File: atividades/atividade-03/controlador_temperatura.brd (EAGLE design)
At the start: 68.6 x 53.3 mm, 34 parts, among them Q1 BC337, Q2 BC337, Q3 BC337

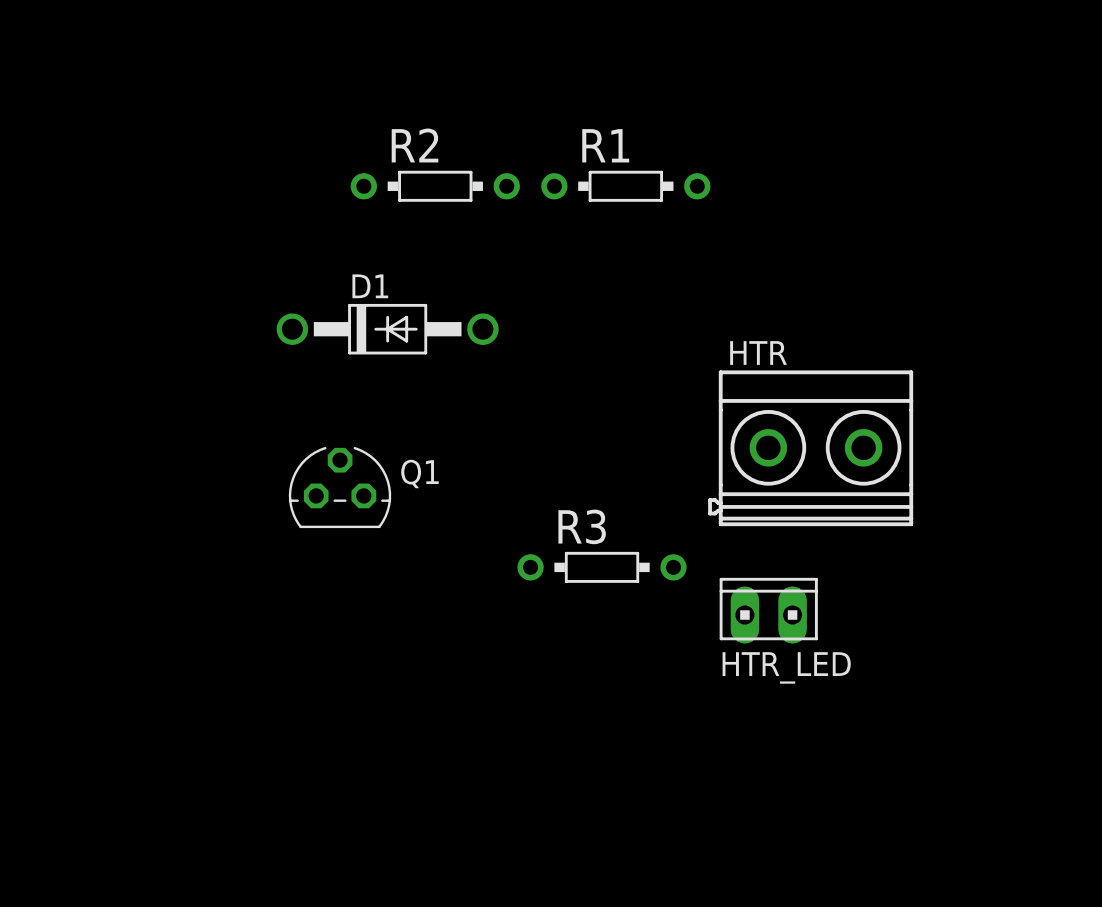
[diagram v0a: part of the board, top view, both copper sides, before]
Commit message: heater realinhado
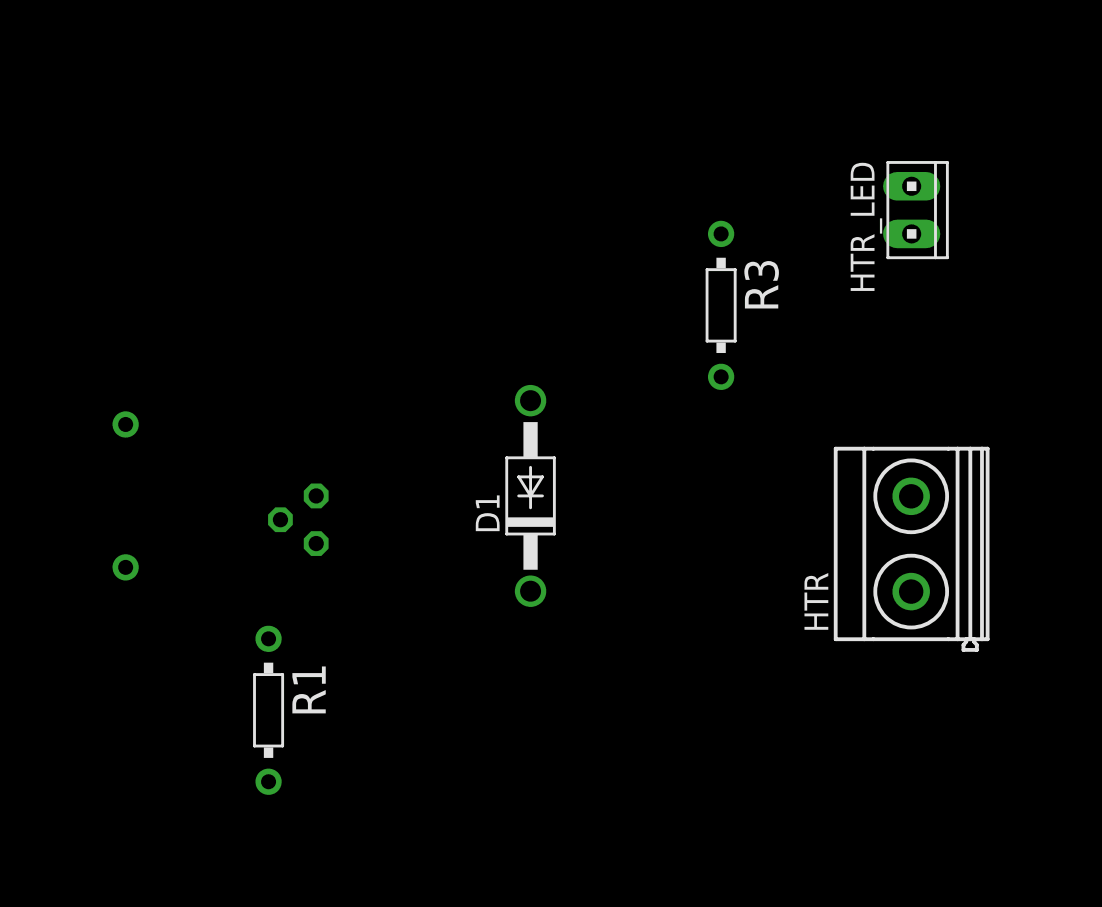
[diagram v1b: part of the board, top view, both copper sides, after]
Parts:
- moved R1 33.8 mm to (-118.1, 111.8), turned to 270 degrees
- moved R2 23.3 mm to (-125.7, 123.2), flipped to the bottom, turned to 270 degrees
- moved HTR_LED 22.9 mm to (-83.8, 138.4), turned to 270 degrees
- moved R3 15.3 mm to (-94.0, 133.3), turned to 270 degrees
- moved D1 11.7 mm to (-104.1, 123.2), turned to 90 degrees
- moved HTR 7.18 mm to (-83.8, 120.7), turned to 90 degrees
- moved Q1 1.80 mm to (-115.6, 121.9), flipped to the bottom, turned to 270 degrees
